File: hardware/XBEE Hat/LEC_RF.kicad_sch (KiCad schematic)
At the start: 8 parts, among them J2 Conn_01x04, U1 XBP9X-DMUS-001, U2 TLV1117LV33DCYR

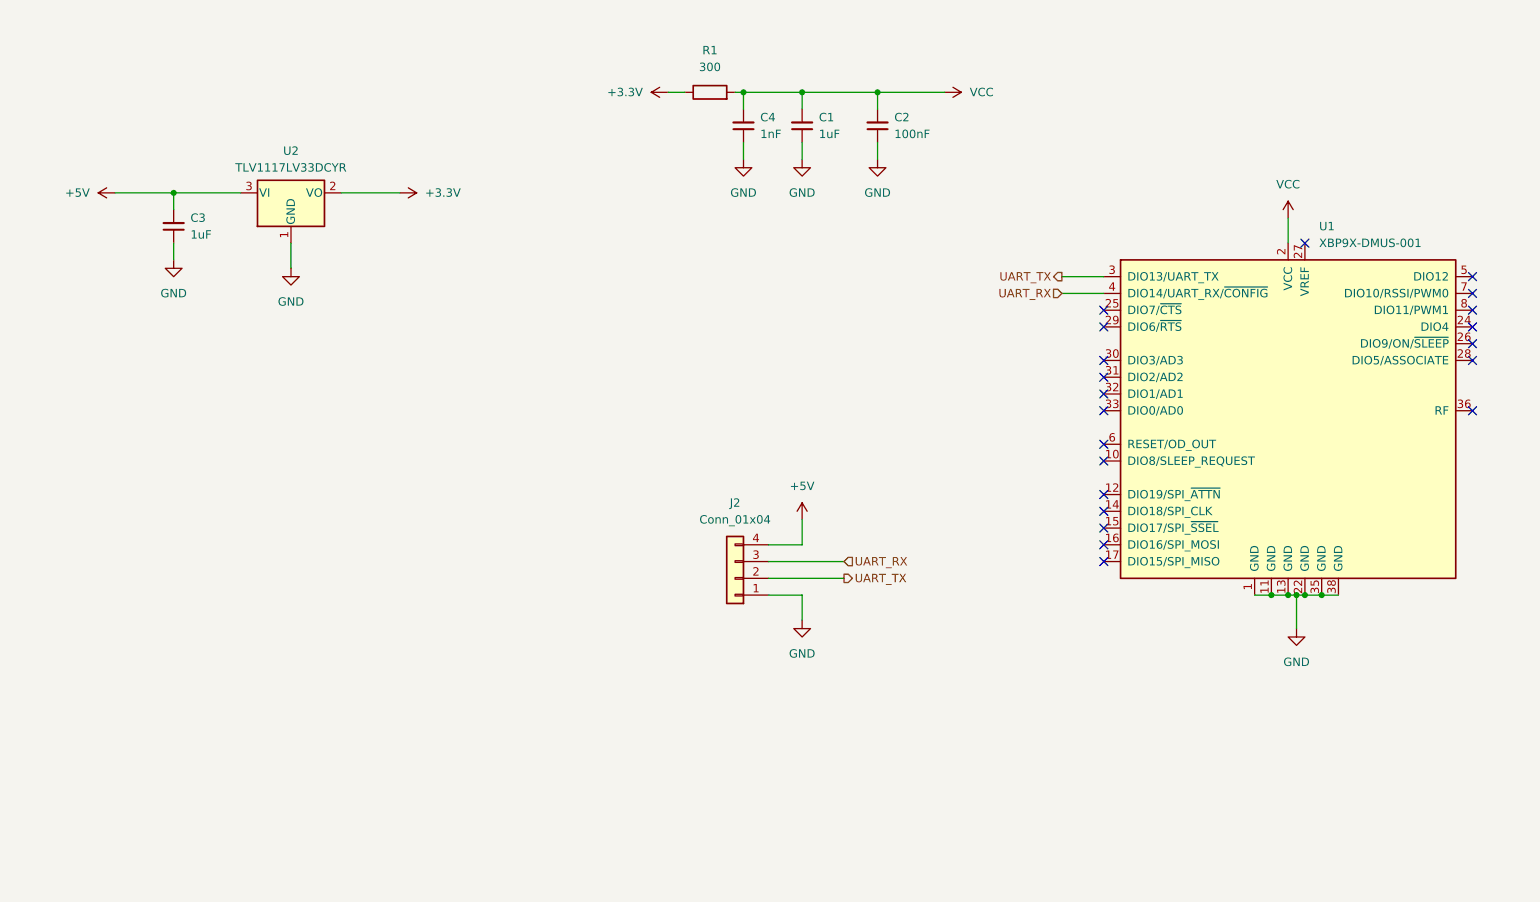
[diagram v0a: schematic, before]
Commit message: Done
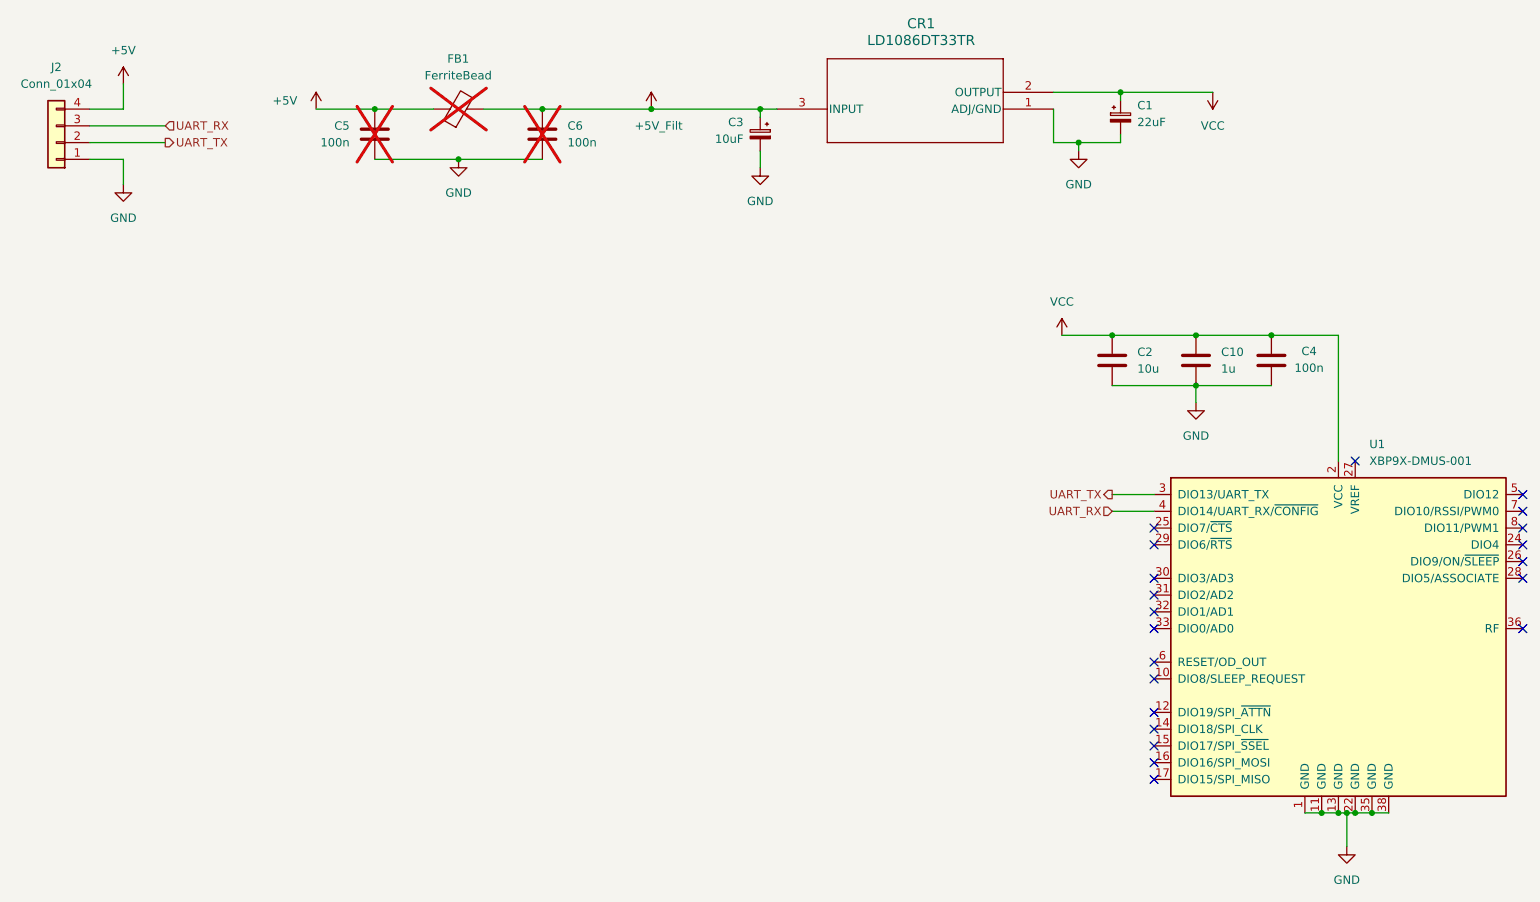
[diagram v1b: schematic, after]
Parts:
- removed C1, C3: 1uF, Capacitor_SMD:C_0805_2012Metric, symbol Device:C_Small
- removed C2: 100nF, Capacitor_SMD:C_0603_1608Metric, symbol Device:C_Small
- removed C4: 1nF, Capacitor_SMD:C_0805_2012Metric, symbol Device:C_Small
- removed R1: 300, Resistor_SMD:R_0805_2012Metric, symbol Device:R
- removed U2: TLV1117LV33DCYR, Package_TO_SOT_SMD:SOT-223-3_TabPin2, symbol Regulator_Linear:TLV1117-33
- added C1: 22uF, Capacitor_SMD:C_0805_2012Metric, symbol Device:C_Polarized_Small
- added C10: 1u, Capacitor_SMD:C_0805_2012Metric, symbol Device:C
- added C2: 10u, Capacitor_SMD:C_1210_3225Metric, symbol Device:C
- added C3: 10uF, Capacitor_SMD:C_0805_2012Metric, symbol Device:C_Polarized_Small
- added C4, C5, C6: 100n, Capacitor_SMD:C_0603_1608Metric, symbol Device:C
- added CR1: LD1086DT33TR, Package_TO_SOT_SMD:TO-252-2, symbol LD1086DT33TR:LD1086DT33TR
- added FB1: FerriteBead, Resistor_SMD:R_0603_1608Metric, symbol Device:FerriteBead
- U1: DigiKey (none) -> https://www.digikey.com/en/products/detail/digi/XBP9X-DMUS-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
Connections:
- net +5V: now also C5.2, FB1.1
- net GND: now also C1.2, C10.2, C2.2, C3.2, C4.1, C5.1, C6.1, CR1.1 (ADJ/GND)
- net VCC: now also C1.1, C10.1, C2.1, C4.2, CR1.2 (OUTPUT)
- new net +5V_Filt: C3.1, C6.2, CR1.3 (INPUT), FB1.2
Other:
- moved on the sheet: J2, U1
